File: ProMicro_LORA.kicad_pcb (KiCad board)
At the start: 2 copper layers, 17.8 x 30.5 mm, 44 parts, among them J1 SMA, J2 COAX, U1 SX1276, U2 AS179-92LF, Y1 32Mhz

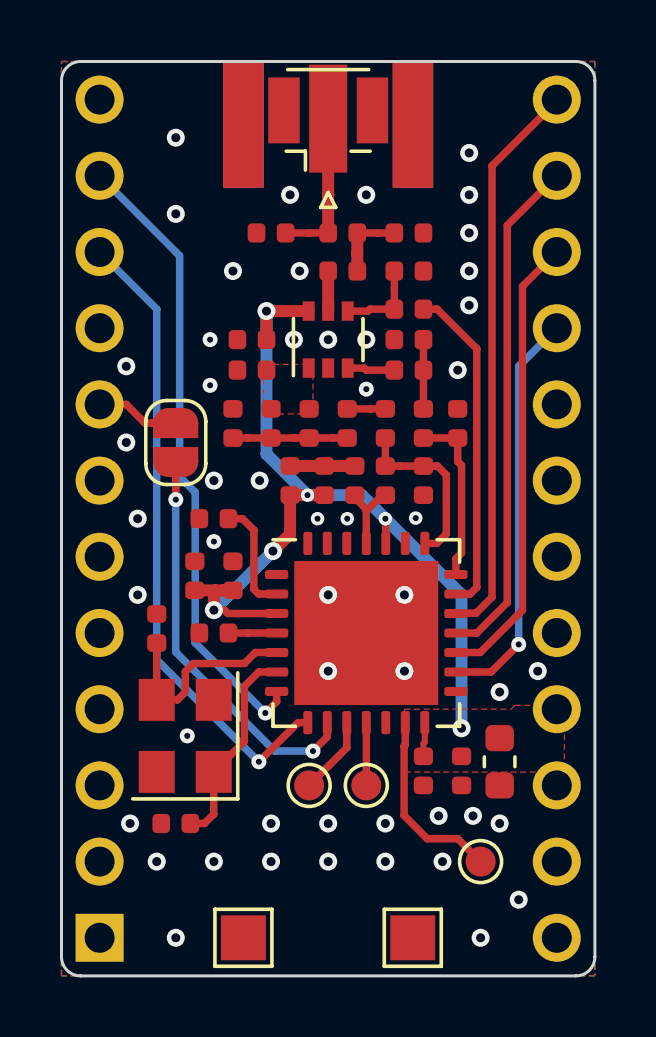
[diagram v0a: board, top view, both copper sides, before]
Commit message: kicad-exports
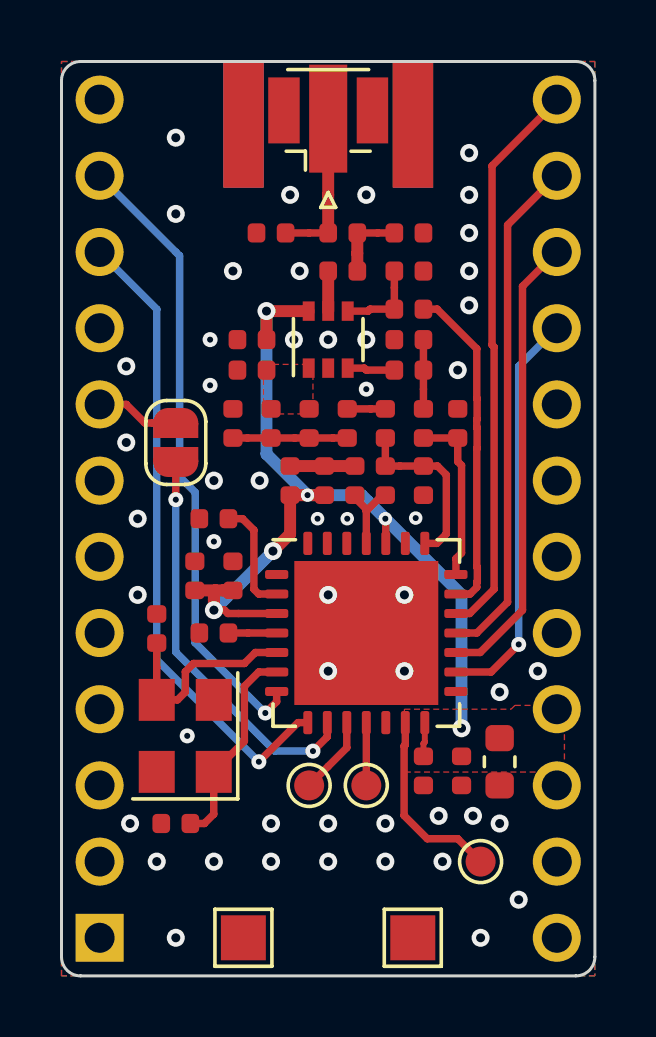
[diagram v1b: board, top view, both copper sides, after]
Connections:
- net MISO renamed D14
- net MOSI renamed D16
- net SCK renamed D15
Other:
- board text added: "CIPO"
- board text added: "CLK"
- board text added: "COPI"
- board text removed: "MISO"
- board text removed: "MOSI"
- board text removed: "SCK"
